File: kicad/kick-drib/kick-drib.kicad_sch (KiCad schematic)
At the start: 23 parts, among them J1 drib-kick, J2 Conn_01x03, J3 drib-kick_POWER, J4 DribblerMotor, J5 Kicker1, K1 G5V-1/12V, Q1 NP52N06SLG, U1 TLP152, U2 TLP152, U3 XL6009/HW-432

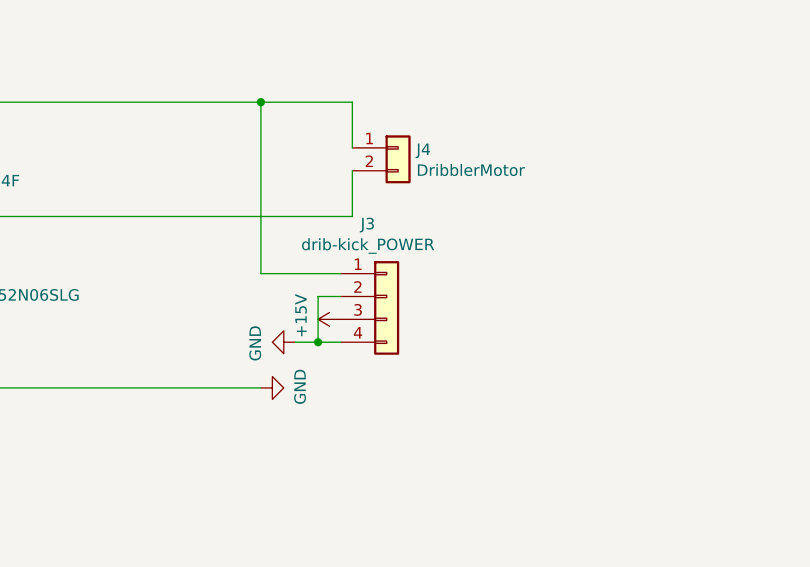
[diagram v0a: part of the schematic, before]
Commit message: fix: main
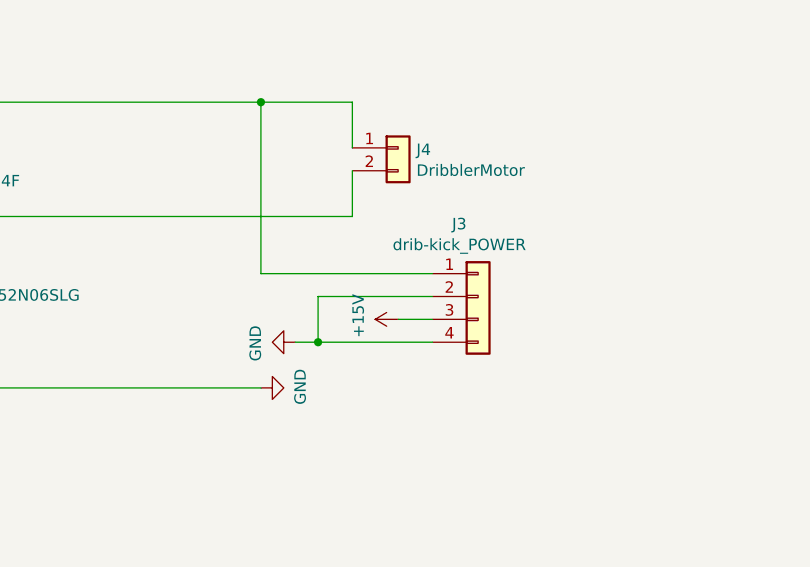
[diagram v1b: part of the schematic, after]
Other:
- moved on the sheet: J3
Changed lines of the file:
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@@
     (stroke (width 0) (type default) (color 0 0 0 0))
   )
-  (wire (pts (xy 167.64 63.5) (xy 176.53 63.5))
+  (wire (pts (xy 167.64 63.5) (xy 186.69 63.5))
     (stroke (width 0) (type default) (color 0 0 0 0))
   )
@@
     (stroke (width 0) (type default) (color 0 0 0 0))
   )
-  (wire (pts (xy 176.53 66.04) (xy 173.99 66.04))
+  (wire (pts (xy 186.69 66.04) (xy 173.99 66.04))
     (stroke (width 0) (type default) (color 0 0 0 0))
   )
@@
     (stroke (width 0) (type default) (color 0 0 0 0))
   )
+  (wire (pts (xy 186.69 68.58) (xy 182.88 68.58))
+    (stroke (width 0) (type default) (color 0 0 0 0))
+  )
   (wire (pts (xy 133.35 184.15) (xy 133.35 196.85))
     (stroke (width 0) (type default) (color 0 0 0 0))
@@
     (stroke (width 0) (type default) (color 0 0 0 0))
   )
-  (wire (pts (xy 173.99 71.12) (xy 176.53 71.12))
+  (wire (pts (xy 173.99 71.12) (xy 186.69 71.12))
     (stroke (width 0) (type default) (color 0 0 0 0))
   )
@@
     (pin "2")
   )
-  (symbol (lib_id "Connector_Generic:Conn_01x04") (at 181.61 66.04 0) (unit 1)
-    (in_bom yes) (on_board yes)
-    (property "Reference" "J3" (id 0) (at 179.5272 57.9882 0))
-    (property "Value" "drib-kick_POWER" (id 1) (at 179.5272 60.2996 0))
-    (property "Footprint" "Connector_PinHeader_2.54mm:PinHeader_1x04_P2.54mm_Vertical" (id 2) (at 181.61 66.04 0)
-      (effects (font (size 1.27 1.27)) hide)
-    )
-    (property "Datasheet" "~" (id 3) (at 181.61 66.04 0)
+  (symbol (lib_id "Connector_Generic:Conn_01x04") (at 191.77 66.04 0) (unit 1)
+    (in_bom yes) (on_board yes)
+    (property "Reference" "J3" (id 0) (at 189.6872 57.9882 0))
+    (property "Value" "drib-kick_POWER" (id 1) (at 189.6872 60.2996 0))
+    (property "Footprint" "Connector_PinHeader_2.54mm:PinHeader_1x04_P2.54mm_Vertical" (id 2) (at 191.77 66.04 0)
+      (effects (font (size 1.27 1.27)) hide)
+    )
+    (property "Datasheet" "~" (id 3) (at 191.77 66.04 0)
       (effects (font (size 1.27 1.27)) hide)
     )
@@
     (pin "2")
   )
-  (symbol (lib_id "power:+15V") (at 176.53 68.58 90) (unit 1)
-    (in_bom yes) (on_board yes)
-    (property "Reference" "#PWR05" (id 0) (at 180.34 68.58 0)
-      (effects (font (size 1.27 1.27)) hide)
-    )
-    (property "Value" "+15V" (id 1) (at 172.1358 68.199 0))
-    (property "Footprint" "" (id 2) (at 176.53 68.58 0)
-      (effects (font (size 1.27 1.27)) hide)
-    )
-    (property "Datasheet" "" (id 3) (at 176.53 68.58 0)
-      (effects (font (size 1.27 1.27)) hide)
-    )
+  (symbol (lib_id "power:+15V") (at 182.88 68.58 90) (unit 1)
+    (in_bom yes) (on_board yes)
+    (property "Reference" "#PWR05" (id 0) (at 186.69 68.58 0)
+      (effects (font (size 1.27 1.27)) hide)
+    )
+    (property "Value" "+15V" (id 1) (at 178.4858 68.199 0))
+    (property "Footprint" "" (id 2) (at 182.88 68.58 0)
+      (effects (font (size 1.27 1.27)) hide)
+    )
+    (property "Datasheet" "" (id 3) (at 182.88 68.58 0)
+      (effects (font (size 1.27 1.27)) hide)
+    )
